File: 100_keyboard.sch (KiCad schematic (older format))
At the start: 40 parts, among them J1 Conn_01x04, J2 Conn_01x03, SW1 SW_Push, U1 mp2359, U2 STM32F072RBTx

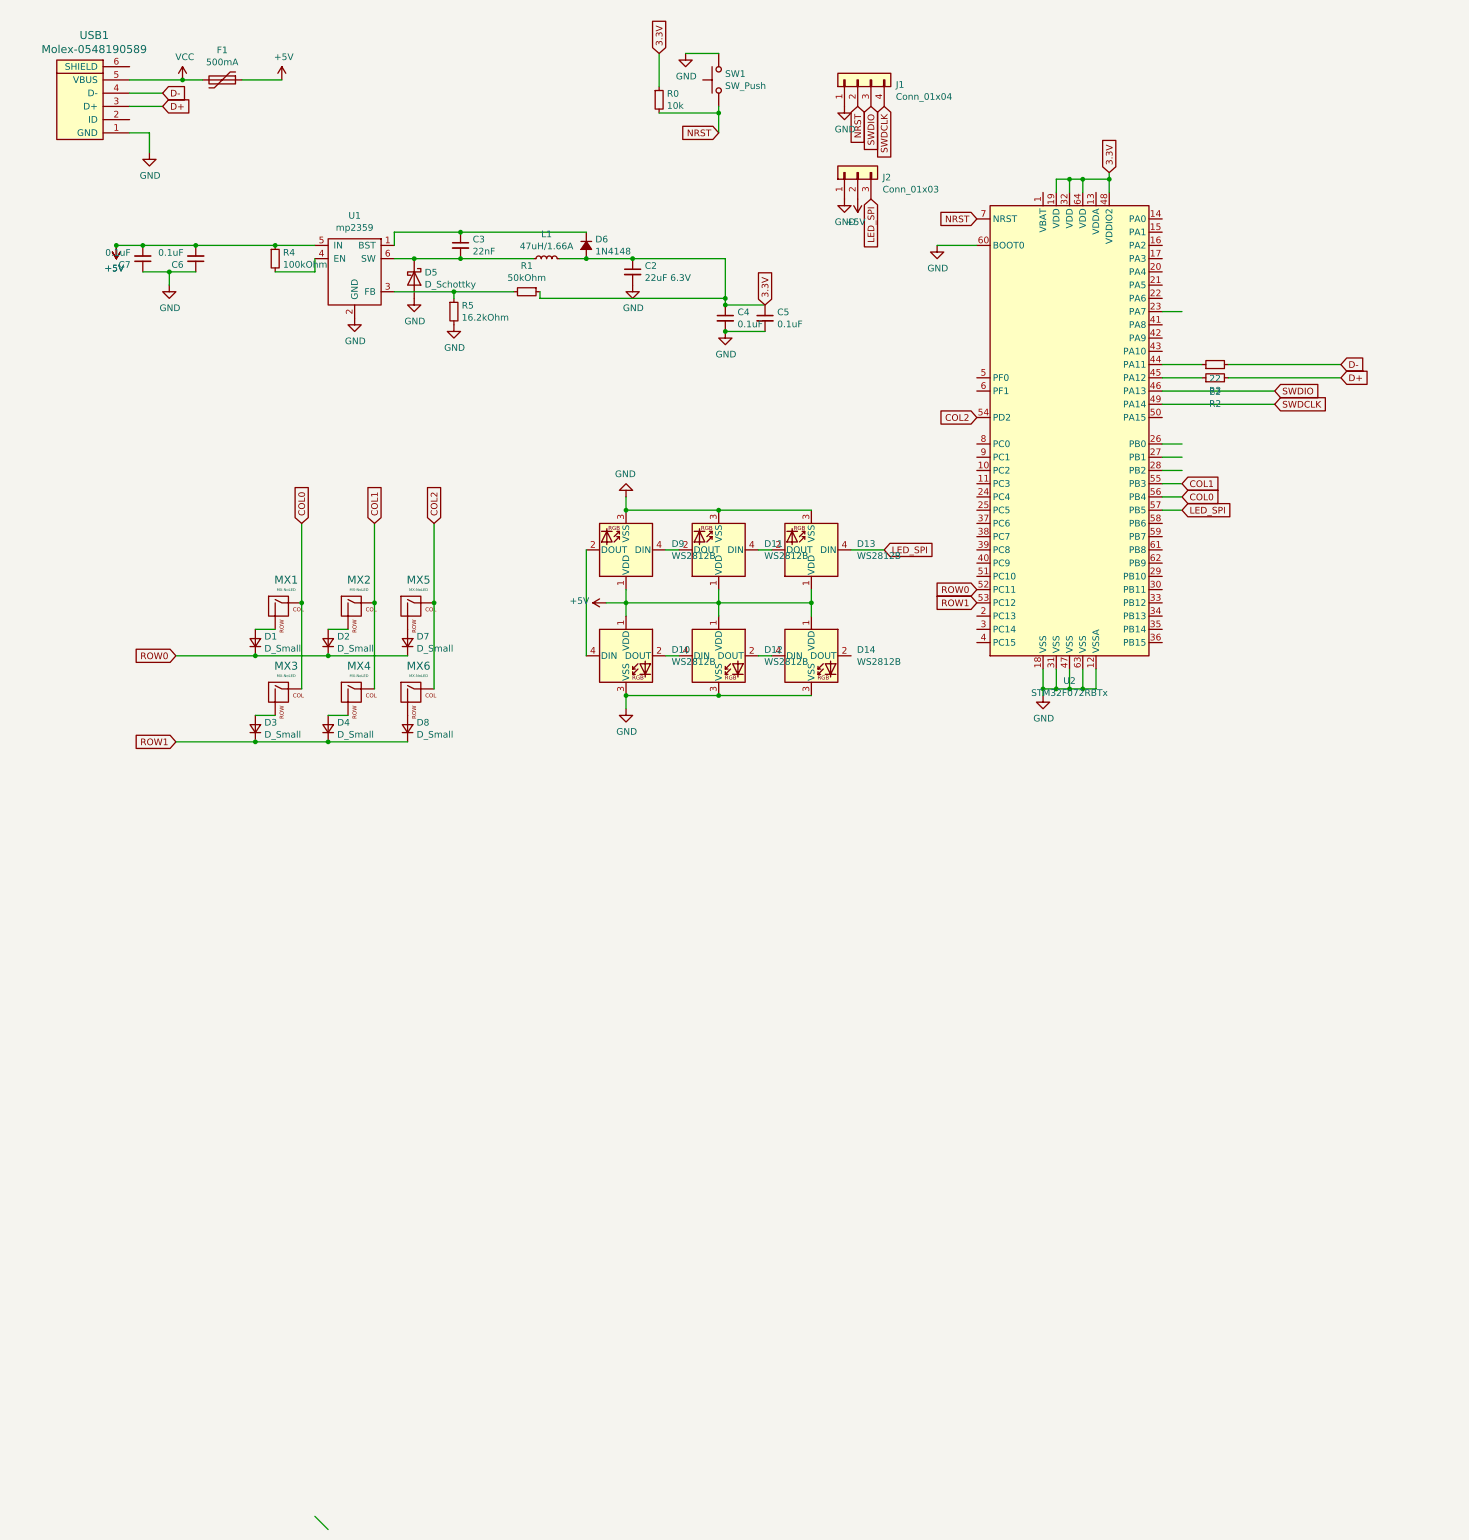
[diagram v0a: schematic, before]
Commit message: Rev 0.4 schematic
Signed-off-by: localcc <work@zloserver.com>
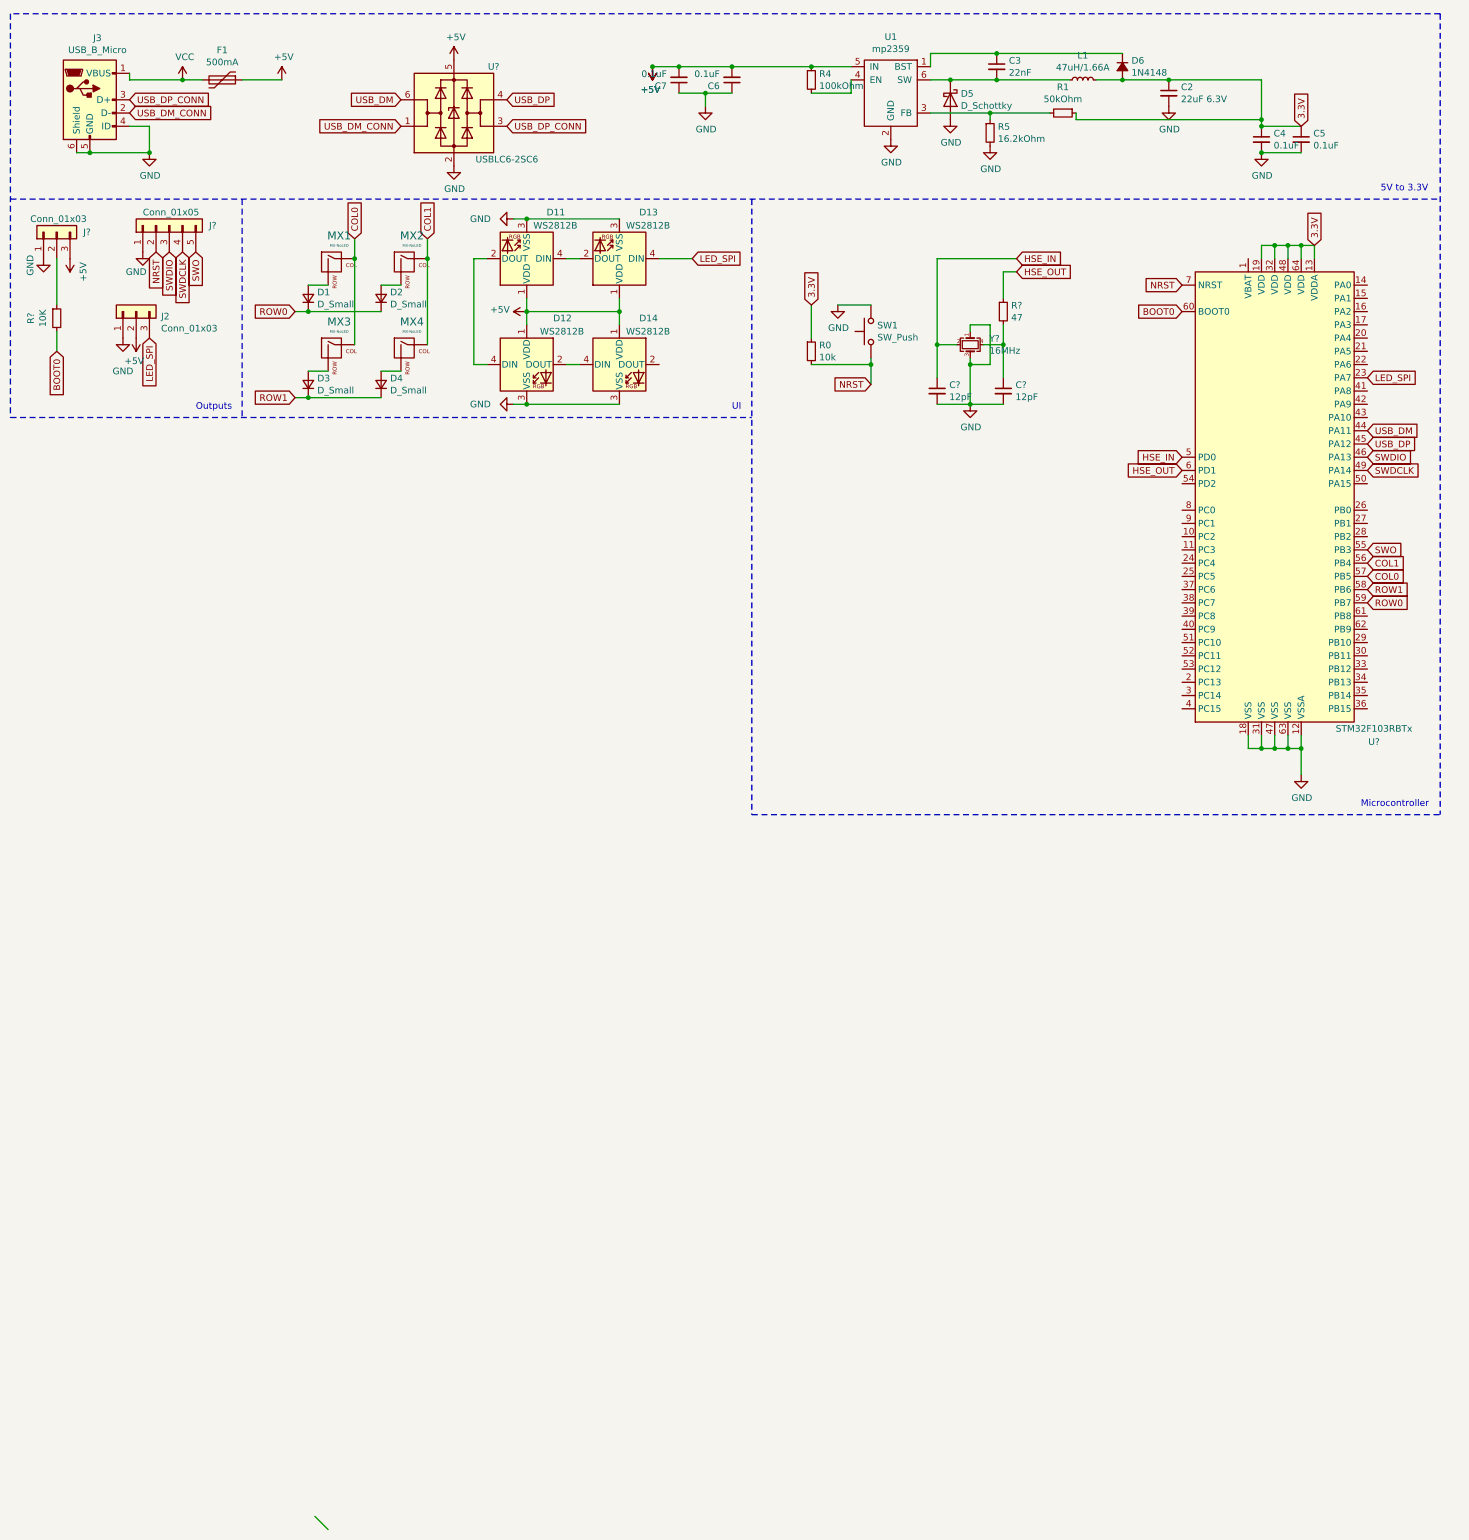
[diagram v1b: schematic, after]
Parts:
- removed D10, D9: WS2812B, LED_SMD:LED_WS2812B_PLCC4_5.0x5.0mm_P3.2mm, symbol LED:WS2812B
- removed D7, D8: D_Small, Diode_SMD:D_SOD-123, symbol Device:D_Small
- removed J1: Conn_01x04, Connector_PinHeader_2.54mm:PinHeader_1x04_P2.54mm_Vertical, symbol Connector_Generic:Conn_01x04
- removed MX5, MX6: MX-NoLED, MX_Alps_Hybrid:MX-1U, symbol 100_keyboard-rescue:MX-NoLED-MX_Alps_Hybrid
- removed R2, R3: 22, Resistor_SMD:R_0805_2012Metric, symbol Device:R_Small
- removed U2: STM32F072RBTx, Package_QFP:LQFP-64_10x10mm_P0.5mm, symbol MCU_ST_STM32F0:STM32F072RBTx
- removed USB1: Molex-0548190589, random-keyboard-parts:Molex-0548190589, symbol 100_keyboard-rescue:Molex-0548190589-random-keyboard-parts
- added C? (x2): 12pF, symbol Device:C_Small
- added J3: USB_B_Micro, Connector_USB:USB_Micro-B_Molex_47346-0001, symbol Connector:USB_B_Micro
- added J?: Conn_01x03, symbol Connector_Generic:Conn_01x03
- added J?: Conn_01x05, symbol Connector_Generic:Conn_01x05
- added R?: 10K, symbol Device:R_Small
- added R?: 47, symbol Device:R_Small
- added U?: STM32F103RBTx, Package_QFP:LQFP-64_10x10mm_P0.5mm, symbol MCU_ST_STM32F1:STM32F103RBTx
- added U?: USBLC6-2SC6, Package_TO_SOT_SMD:SOT-23-6, symbol Power_Protection:USBLC6-2SC6
- added Y?: 16MHz, symbol Device:Crystal_GND24_Small
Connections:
- net labels added: BOOT0, HSE_IN, HSE_OUT, SWO, USB_DM, USB_DM_CONN, USB_DP, USB_DP_CONN
- net labels removed: COL2, D+, D-
- wire segments 108 -> 105
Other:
- note added: "5V to 3.3V\n"
- note added: "Microcontroller\n"
- note added: "Outputs\n"
- note added: "UI\n"
- moved on the sheet: C2, C3, C4, C5, C6, C7, D1, D11, D12, D13, D14, D2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
